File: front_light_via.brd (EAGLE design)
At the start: 48.7 x 79.1 mm, 9 parts

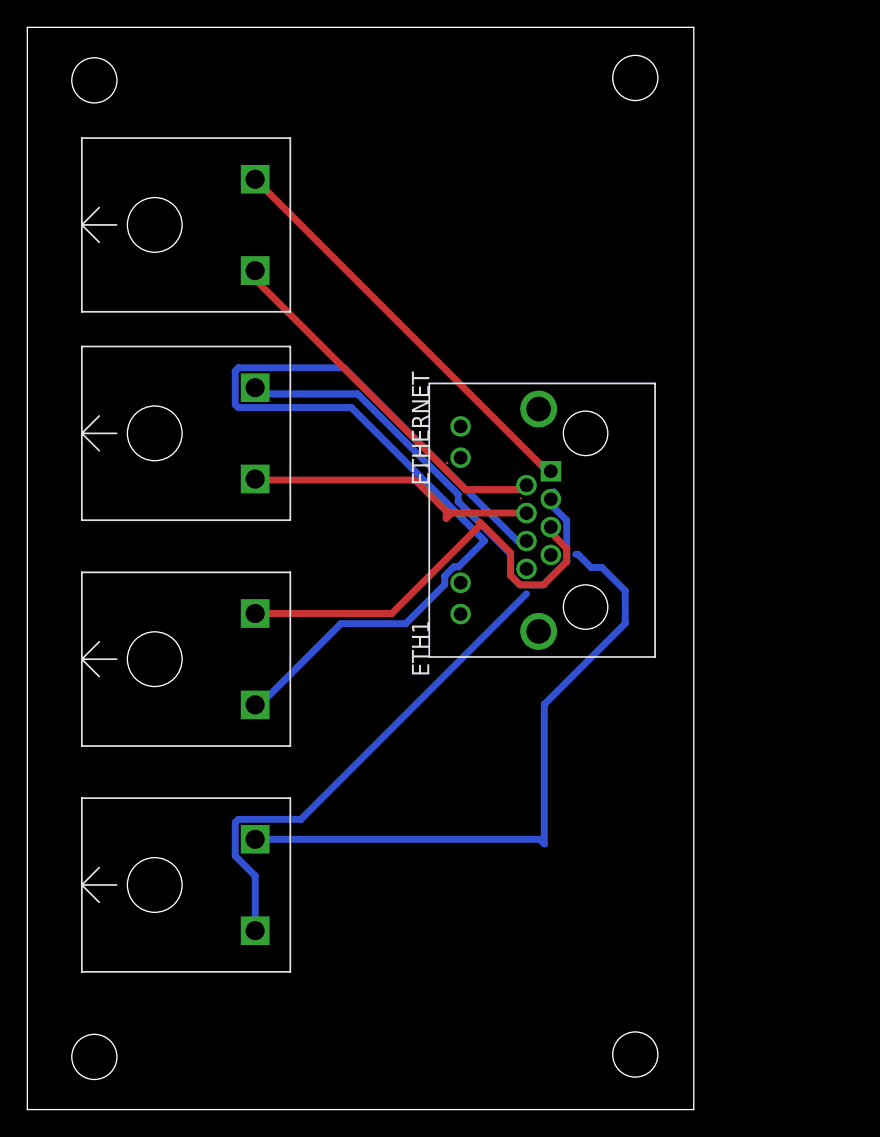
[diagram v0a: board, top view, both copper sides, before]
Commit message: via gerbers generated
via boards completed and gerbers generated
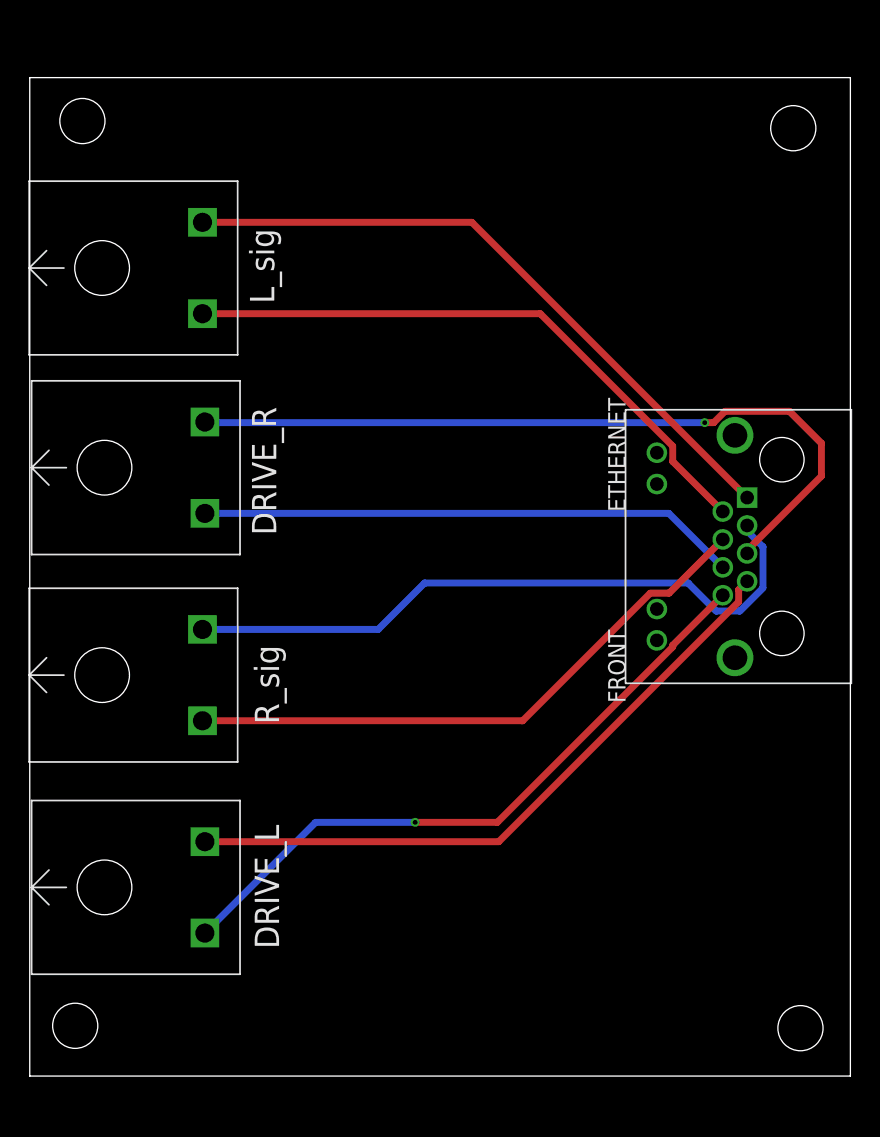
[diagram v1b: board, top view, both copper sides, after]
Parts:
- removed ETH1: ETHERNET, ETHERNET:A122645-ND
- removed L_DRIVE, L_SIG, R-DRIVE, R_SIG: 2_PIN_TECONNECTOR, TE 2-pin connector:2_PIN_CONNECT
- added BLINK_L, BLINK_R, DRIVING_L, DRIVING_R: 2_PIN_TECONNECTOR, TE 2-pin connector:2_PIN_CONNECT
- added FRONT: ETHERNET, ETHERNET:A122645-ND
- moved H2 12.2 mm to (56.4, 3.50)
- moved H4 12.1 mm to (55.8, 69.3)
- moved H3 3.10 mm to (3.85, 69.8)
- moved H1 2.67 mm to (3.33, 3.67)
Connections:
- removed net N$2: ETH1.P$2, R-DRIVE.G/LOW
- removed net N$4: ETH1.P$4, L_DRIVE.G/LOW
- removed net N$6: ETH1.P$6, R_SIG.G/LOW
- removed net N$8: ETH1.P$8, L_SIG.G/LOW
- new net BLIINK_R: BLINK_R.G/LOW, FRONT.P$4
- new net BLINK_L: BLINK_L.G/LOW, FRONT.P$2
- new net DRIVING_L: DRIVING_L.G/LOW, FRONT.P$8
- new net DRIVING_R: DRIVING_R.G/LOW, FRONT.P$6
- net N$1: now also BLINK_L.V/SIG, FRONT.P$1; no longer ETH1.P$1, R-DRIVE.V/SIG
- net N$3: now also BLINK_R.V/SIG, FRONT.P$3; no longer ETH1.P$3, L_DRIVE.V/SIG
- net N$5: now also DRIVING_R.V/SIG, FRONT.P$5; no longer ETH1.P$5, R_SIG.V/SIG
- net N$7: now also DRIVING_L.V/SIG, FRONT.P$7; no longer ETH1.P$7, L_SIG.V/SIG
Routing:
- net N$6: track 73.5 -> 0.00 mm
- net DRIVING_L: track 0.00 -> 48.2 mm, vias 0 -> 1
- net BLINK_L: track 0.00 -> 44.7 mm
- net BLIINK_R: track 0.00 -> 43.5 mm
- net DRIVING_R: track 0.00 -> 39.5 mm
- net N$8: track 36.7 -> 0.00 mm
- net N$2: track 27.0 -> 0.00 mm
- net N$5: track 33.4 -> 56.7 mm, vias 0 -> 1
- net N$4: track 21.5 -> 0.00 mm
- net N$1: track 30.7 -> 48.2 mm
- net N$3: track 36.9 -> 49.0 mm
- net N$7: track 47.0 -> 48.0 mm
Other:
- board size 48.7 x 79.1 mm -> 60 x 73 mm
- board text added: "DRIVE_L"
- board text added: "DRIVE_R"
- board text added: "L_sig"
- board text added: "R_sig"
